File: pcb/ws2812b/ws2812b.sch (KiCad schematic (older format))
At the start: 19 parts, among them J1 Jack-DC, J2 Conn_02x08_Top_Bottom, J3 Conn_01x02, J4 Conn_02x08_Top_Bottom, J5 Conn_01x08, J6 Conn_01x08, J7 Conn_01x08, J8 Conn_01x02, U1 AMS1117-3.3, U2 STM32F103C8Tx, U3 74HC245

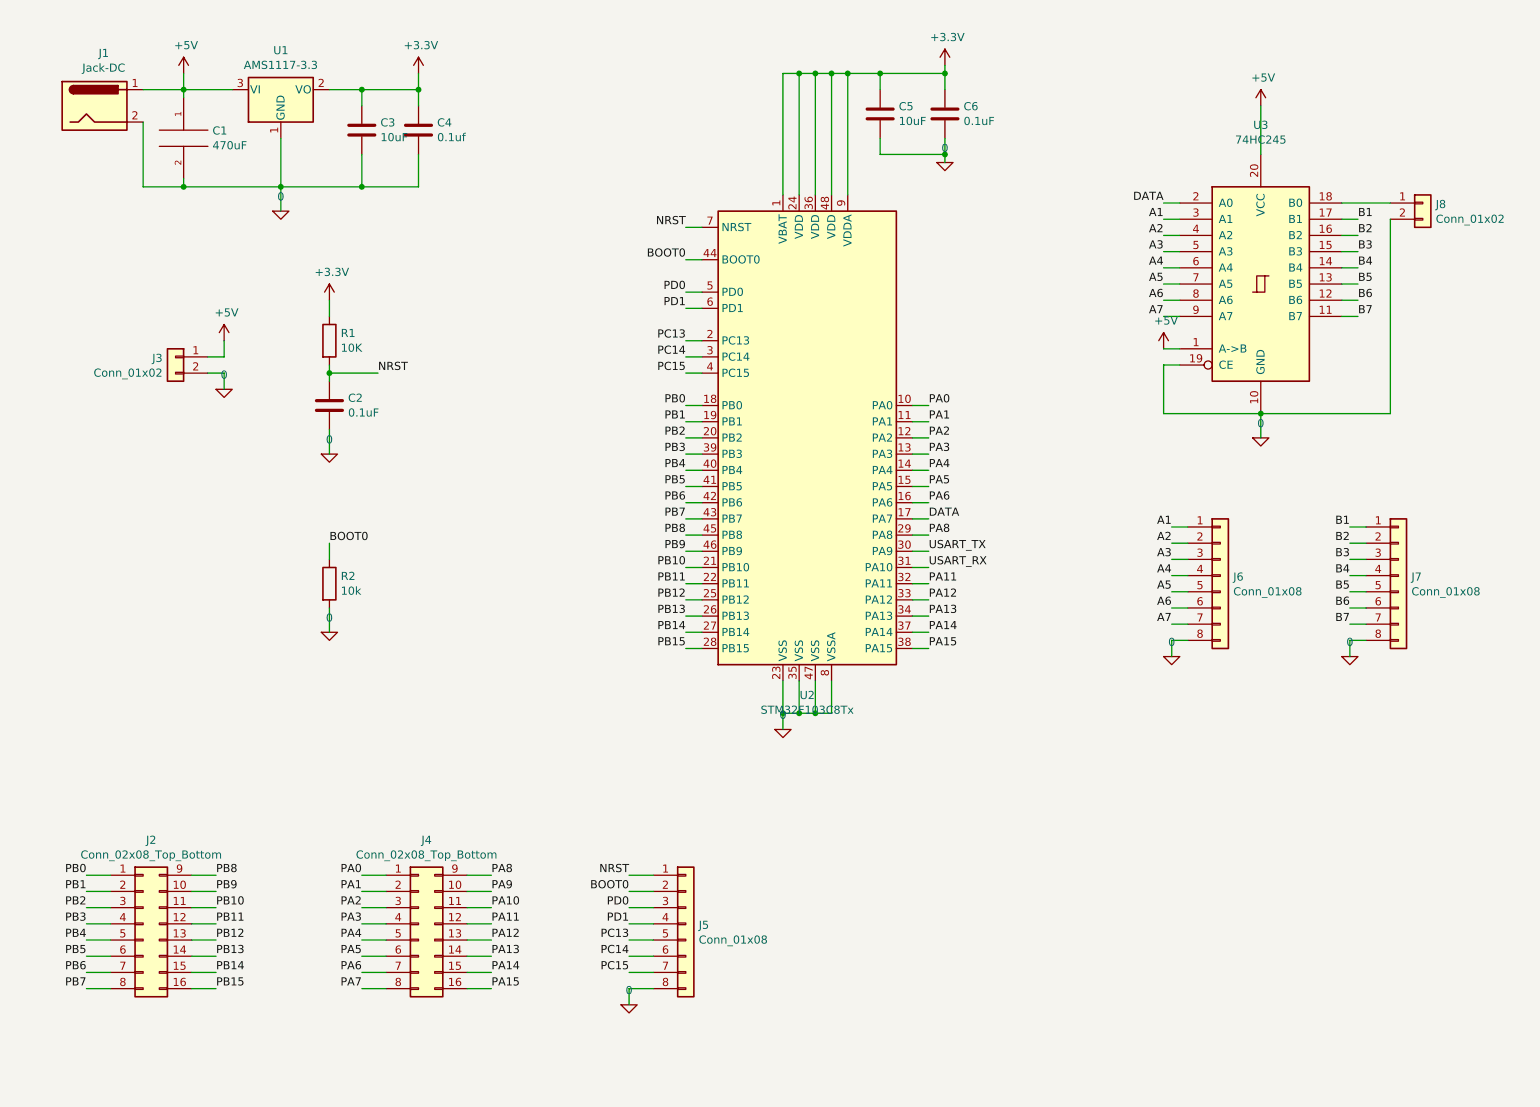
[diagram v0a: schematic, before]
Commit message: 20190425
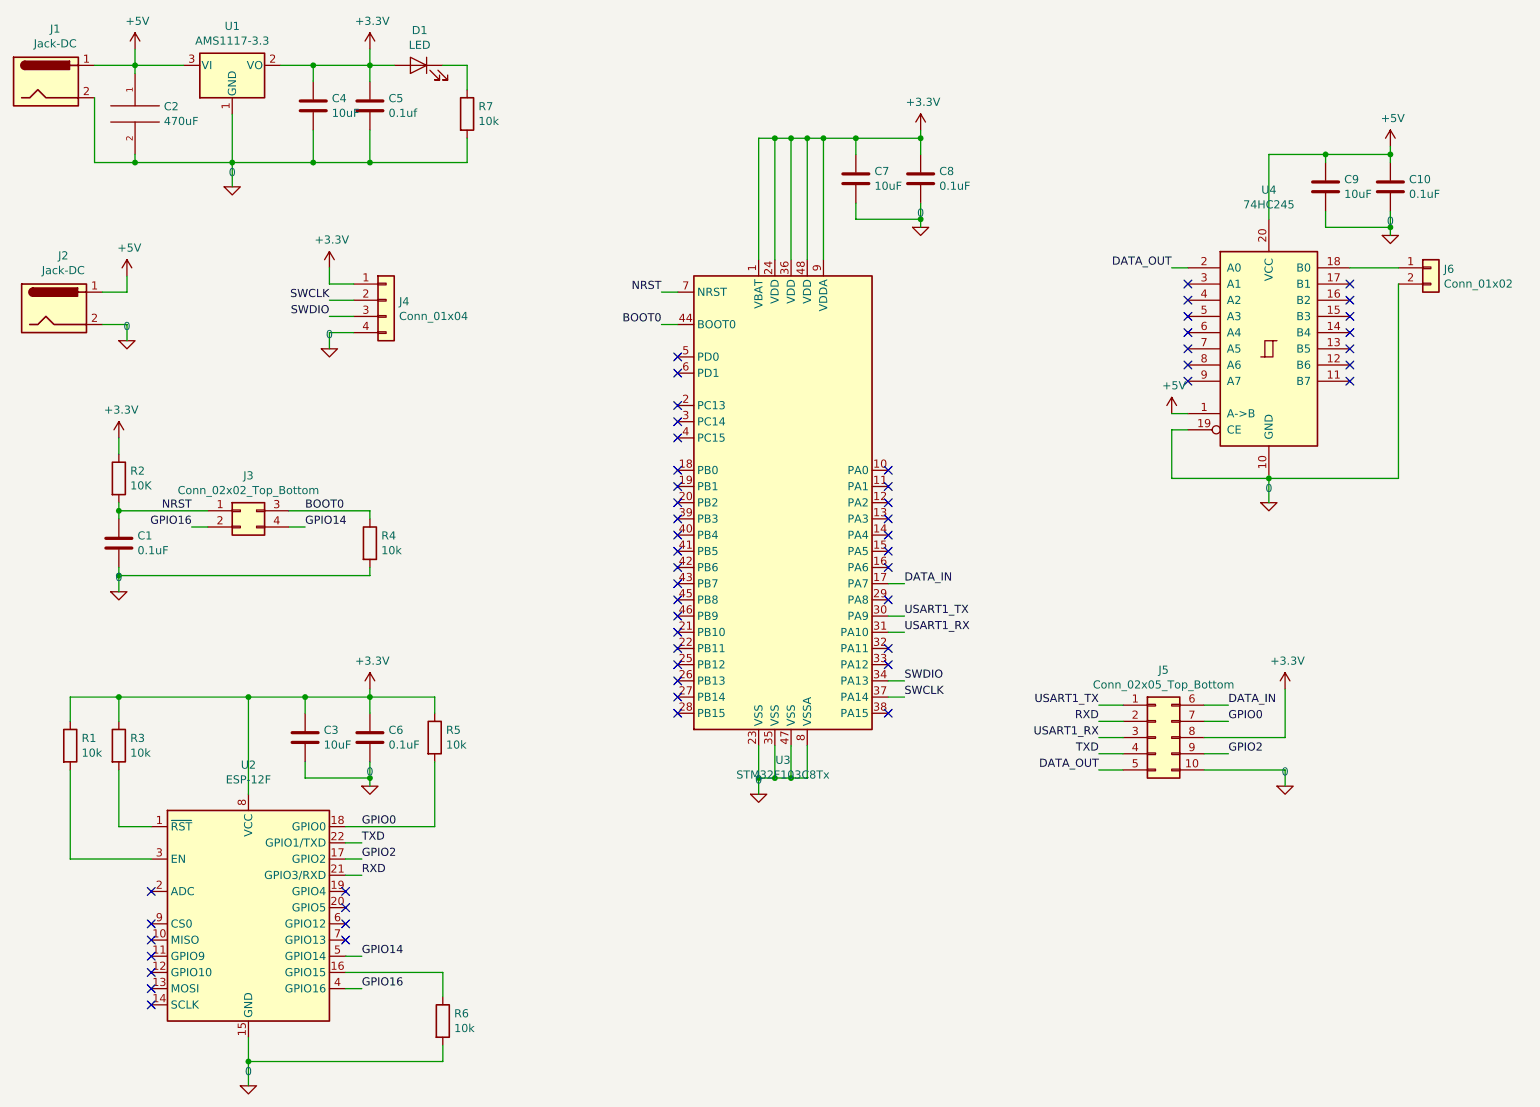
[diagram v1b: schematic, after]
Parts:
- removed J2, J4: Conn_02x08_Top_Bottom, Connector_PinHeader_2.54mm:PinHeader_2x08_P2.54mm_Vertical, symbol Connector_Generic:Conn_02x08_Top_Bottom
- removed J3: Conn_01x02, Connector_PinHeader_2.54mm:PinHeader_1x02_P2.54mm_Vertical, symbol Connector_Generic:Conn_01x02
- removed J5, J6, J7: Conn_01x08, Connector_PinHeader_2.54mm:PinHeader_1x08_P2.54mm_Vertical, symbol Connector_Generic:Conn_01x08
- added C10, C6: 0.1uF, Capacitor_SMD:C_0805_2012Metric_Pad1.15x1.40mm_HandSolder, symbol Device:C
- added C3, C9: 10uF, Capacitor_SMD:C_0805_2012Metric_Pad1.15x1.40mm_HandSolder, symbol Device:C
- added D1: LED, LED_SMD:LED_0805_2012Metric_Pad1.15x1.40mm_HandSolder, symbol Device:LED
- added J2: Jack-DC, Connector_BarrelJack:BarrelJack_Horizontal, symbol Connector:Jack-DC
- added J3: Conn_02x02_Top_Bottom, Connector_PinHeader_2.54mm:PinHeader_2x02_P2.54mm_Vertical, symbol Connector_Generic:Conn_02x02_Top_Bottom
- added J4: Conn_01x04, Connector_PinHeader_2.54mm:PinHeader_1x04_P2.54mm_Vertical, symbol Connector_Generic:Conn_01x04
- added J5: Conn_02x05_Top_Bottom, Connector_PinHeader_2.54mm:PinHeader_2x05_P2.54mm_Vertical, symbol Connector_Generic:Conn_02x05_Top_Bottom
- added R1, R3, R5, R6, R7: 10k, Resistor_SMD:R_0805_2012Metric_Pad1.15x1.40mm_HandSolder, symbol Device:R
- added U2: ESP-12F, RF_Module:ESP-12E, symbol RF_Module:ESP-12F
- U1: footprint Package_TO_SOT_SMD:SOT-223-3_TabPin2 -> Package_TO_SOT_SMD:SOT-223
- renumbered C2 to C1, C1 to C2, C3 to C4, C4 to C5, C5 to C7, C6 to C8, J8 to J6, R1 to R2, R2 to R4, U2 to U3, U3 to U4
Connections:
- net +3V3: now also C3.1, C6.1, D1.2 (A), J4.1 (Pin_1), J5.8 (Pin_8), R1.1, R3.1, R5.1, U2.8 (VCC)
- net +5V: now also C10.1, C9.1, J2.1
- net 0: now also C10.2, C3.2, C6.2, C9.2, J2.2, J4.4 (Pin_4), J5.10 (Pin_10), R6.2, R7.2, U2.15 (GND)
- net BOOT0: now also J3.3 (Pin_3)
- net NRST: now also J3.1 (Pin_1)
- net A1: no longer names the net of U4.3 (A1)
- net A2: no longer names the net of U4.4 (A2)
- net A3: no longer names the net of U4.5 (A3)
- net A4: no longer names the net of U4.6 (A4)
- net A5: no longer names the net of U4.7 (A5)
- net A6: no longer names the net of U4.8 (A6)
- net A7: no longer names the net of U4.9 (A7)
- net B1: no longer names the net of U4.17 (B1)
- net B2: no longer names the net of U4.16 (B2)
- net B3: no longer names the net of U4.15 (B3)
- net B4: no longer names the net of U4.14 (B4)
- net B5: no longer names the net of U4.13 (B5)
- net B6: no longer names the net of U4.12 (B6)
- net B7: no longer names the net of U4.11 (B7)
- net DATA renamed DATA_IN
- net DATA_IN: now also J5.6 (Pin_6); no longer U4.2 (A0)
- net PA0: no longer names the net of U3.10 (PA0)
- net PA1: no longer names the net of U3.11 (PA1)
- net PA11: no longer names the net of U3.32 (PA11)
- net PA12: no longer names the net of U3.33 (PA12)
- net PA13 renamed SWDIO
- net SWDIO: now also J4.3 (Pin_3)
- net PA14 renamed SWCLK
- net SWCLK: now also J4.2 (Pin_2)
- net PA15: no longer names the net of U3.38 (PA15)
- net PA2: no longer names the net of U3.12 (PA2)
- net PA3: no longer names the net of U3.13 (PA3)
- net PA4: no longer names the net of U3.14 (PA4)
- net PA5: no longer names the net of U3.15 (PA5)
- net PA6: no longer names the net of U3.16 (PA6)
- net PA8: no longer names the net of U3.29 (PA8)
- net PB0: no longer names the net of U3.18 (PB0)
- net PB1: no longer names the net of U3.19 (PB1)
- net PB10: no longer names the net of U3.21 (PB10)
- net PB11: no longer names the net of U3.22 (PB11)
- net PB12: no longer names the net of U3.25 (PB12)
- net PB13: no longer names the net of U3.26 (PB13)
- net PB14: no longer names the net of U3.27 (PB14)
- net PB15: no longer names the net of U3.28 (PB15)
- net PB2: no longer names the net of U3.20 (PB2)
- net PB3: no longer names the net of U3.39 (PB3)
- net PB4: no longer names the net of U3.40 (PB4)
- net PB5: no longer names the net of U3.41 (PB5)
- net PB6: no longer names the net of U3.42 (PB6)
- net PB7: no longer names the net of U3.43 (PB7)
- net PB8: no longer names the net of U3.45 (PB8)
- net PB9: no longer names the net of U3.46 (PB9)
- net PC13: no longer names the net of U3.2 (PC13)
- net PC14: no longer names the net of U3.3 (PC14)
- net PC15: no longer names the net of U3.4 (PC15)
- net PD0: no longer names the net of U3.5 (PD0)
- net PD1: no longer names the net of U3.6 (PD1)
- net USART_RX renamed USART1_RX
- net USART1_RX: now also J5.3 (Pin_3)
- net USART_TX renamed USART1_TX
- net USART1_TX: now also J5.1 (Pin_1)
- new net: R3.2, U2.1 (~RST)
- new net: R6.1, U2.16 (GPIO15)
- new net: R1.2, U2.3 (EN)
- new net: D1.1 (K), R7.1
- new net DATA_OUT: J5.5 (Pin_5), U4.2 (A0)
- new net GPIO0: J5.7 (Pin_7), R5.2, U2.18 (GPIO0)
- new net GPIO14: J3.4 (Pin_4), U2.5 (GPIO14)
- new net GPIO16: J3.2 (Pin_2), U2.4 (GPIO16)
- new net GPIO2: J5.9 (Pin_9), U2.17 (GPIO2)
- new net RXD: J5.2 (Pin_2), U2.21 (GPIO3/RXD)
- new net TXD: J5.4 (Pin_4), U2.22 (GPIO1/TXD)
- no-connect marks 0 -> 57
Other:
- moved on the sheet: C1, C2, C4, C5, C7, C8, J1, J6, R2, R4, U1, U3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
